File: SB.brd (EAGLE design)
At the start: 68 x 30 mm, 33 parts, among them IC1 ATMEGA32U4NT-TQFP, J1 USB-6P-SMT, J2 RJ12, J3 AUDIO-JACK-PJ321, J4 NO/NC, K1 HE721C-DIP, Q1 2N7002, Q2 RJU003N03

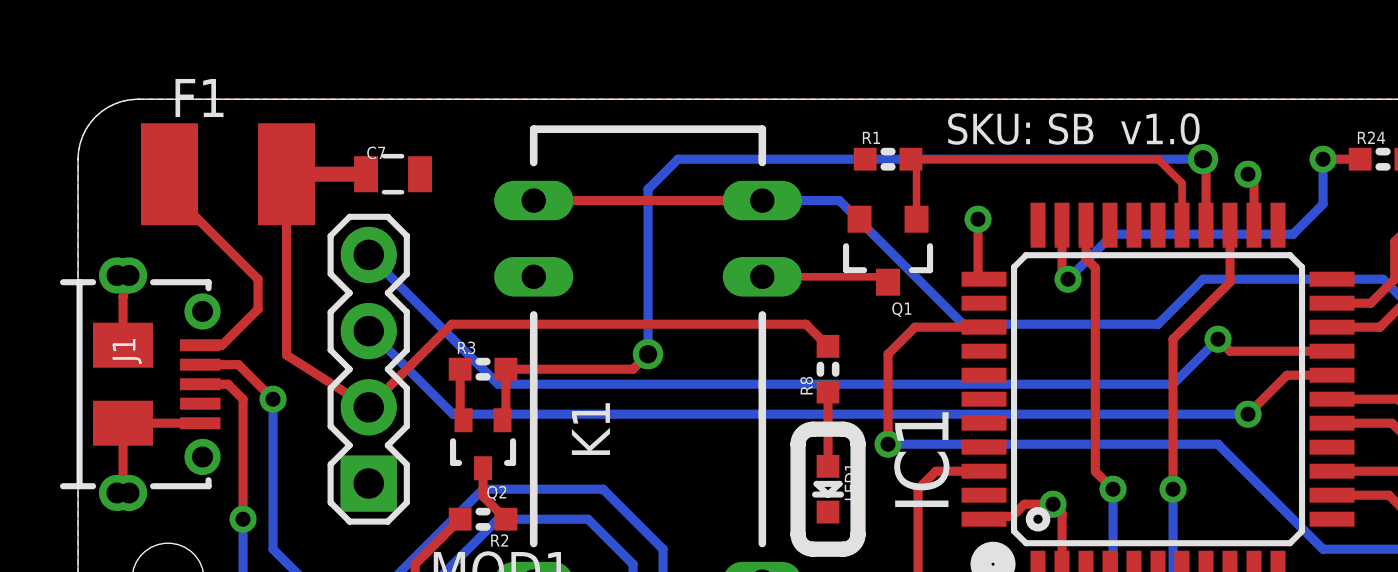
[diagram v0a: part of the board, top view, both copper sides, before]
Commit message: ERC / DRC for v1.0 release
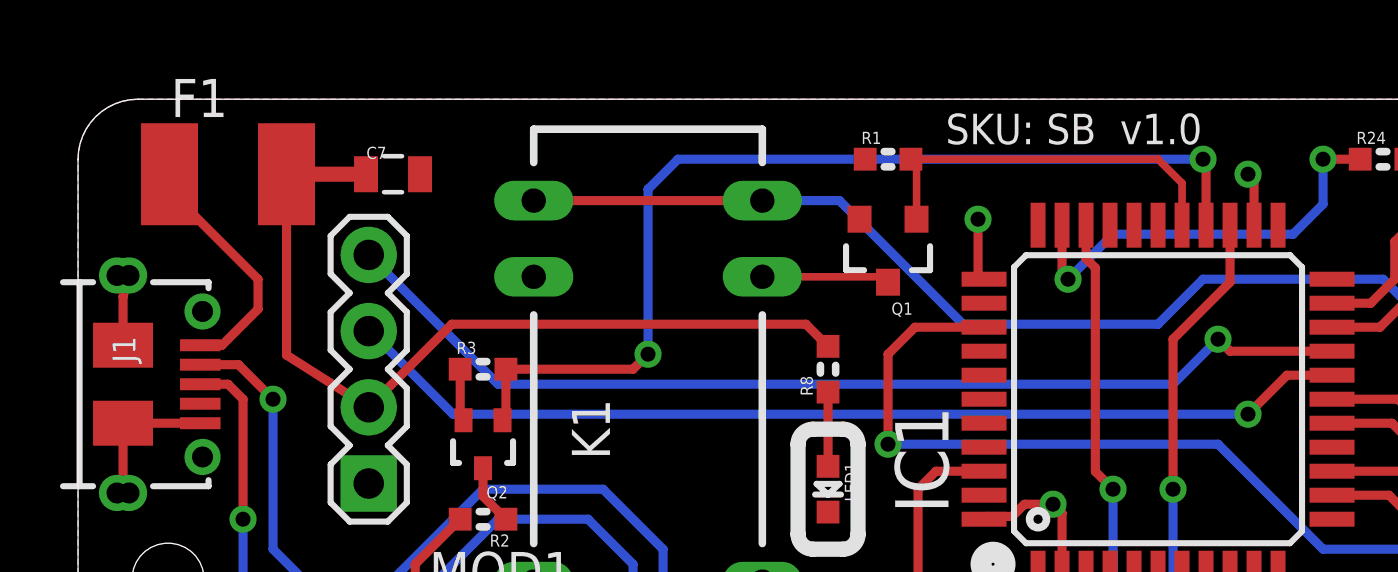
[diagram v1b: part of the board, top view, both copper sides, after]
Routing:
- net USB+: track 8.70 -> 8.14 mm
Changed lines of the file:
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@@
 <?xml version="1.0" encoding="utf-8"?>
 <!DOCTYPE eagle SYSTEM "eagle.dtd">
-<eagle version="9.5.2">
+<eagle version="9.5.1">
 <drawing>
 <settings>
@@
 <signal name="A0">
 <contactref element="IC1" pad="36"/>
-<wire x1="30.2" y1="23.4" x2="30.1072" y2="23.4928" width="0.3048" layer="1"/>
 <wire x1="30.2" y1="23.4" x2="27.9" y2="23.4" width="0.3048" layer="1"/>
 <wire x1="27.9" y1="23.4" x2="27" y2="22.5" width="0.3048" layer="1"/>
@@
 <contactref element="F1" pad="1"/>
 <wire x1="6" y1="24" x2="6" y2="25" width="0.3048" layer="1"/>
-<wire x1="3" y1="27.95" x2="3.05" y2="28.5" width="0.3048" layer="1"/>
 <wire x1="4.075" y1="22.8" x2="4.8" y2="22.8" width="0.3048" layer="1"/>
 <wire x1="4.8" y1="22.8" x2="6" y2="24" width="0.3048" layer="1"/>
@@
 <wire x1="14.262" y1="22" x2="18.5" y2="22" width="0.3048" layer="1"/>
 <wire x1="18.5" y1="22" x2="19" y2="22.5" width="0.3048" layer="1"/>
-<via x="19" y="22.5" extent="1-16" drill="0.6096"/>
+<via x="19" y="22.5" extent="1-16" drill="0.5"/>
 <wire x1="19" y1="22.5" x2="19" y2="28" width="0.3048" layer="16"/>
 <wire x1="20" y1="29" x2="37.5" y2="29" width="0.3048" layer="16"/>
-<via x="37.5" y="29" extent="1-16" drill="0.6096"/>
+<via x="37.5" y="29" extent="1-16" drill="0.5"/>
 <wire x1="37.5" y1="29" x2="37.6" y2="28.9" width="0.3048" layer="1"/>
 <wire x1="37.6" y1="28.9" x2="37.6" y2="26.8" width="0.3048" layer="1"/>
